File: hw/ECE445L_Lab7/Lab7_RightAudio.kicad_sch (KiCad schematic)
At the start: 60 parts, among them Q10 PZT2222A, Q11 PZT2222A, Q12 PZT2222A, Q13 PZT2222A, Q14 PZT2222A, Q15 PZT2222A, Q16 PZT2222A, Q17 PZT2222A, Q18 PZT2222A, U11 OPA2350, U12 OPA2350, U13 OPA2350, U15 TLV5616, U6 OPA2350

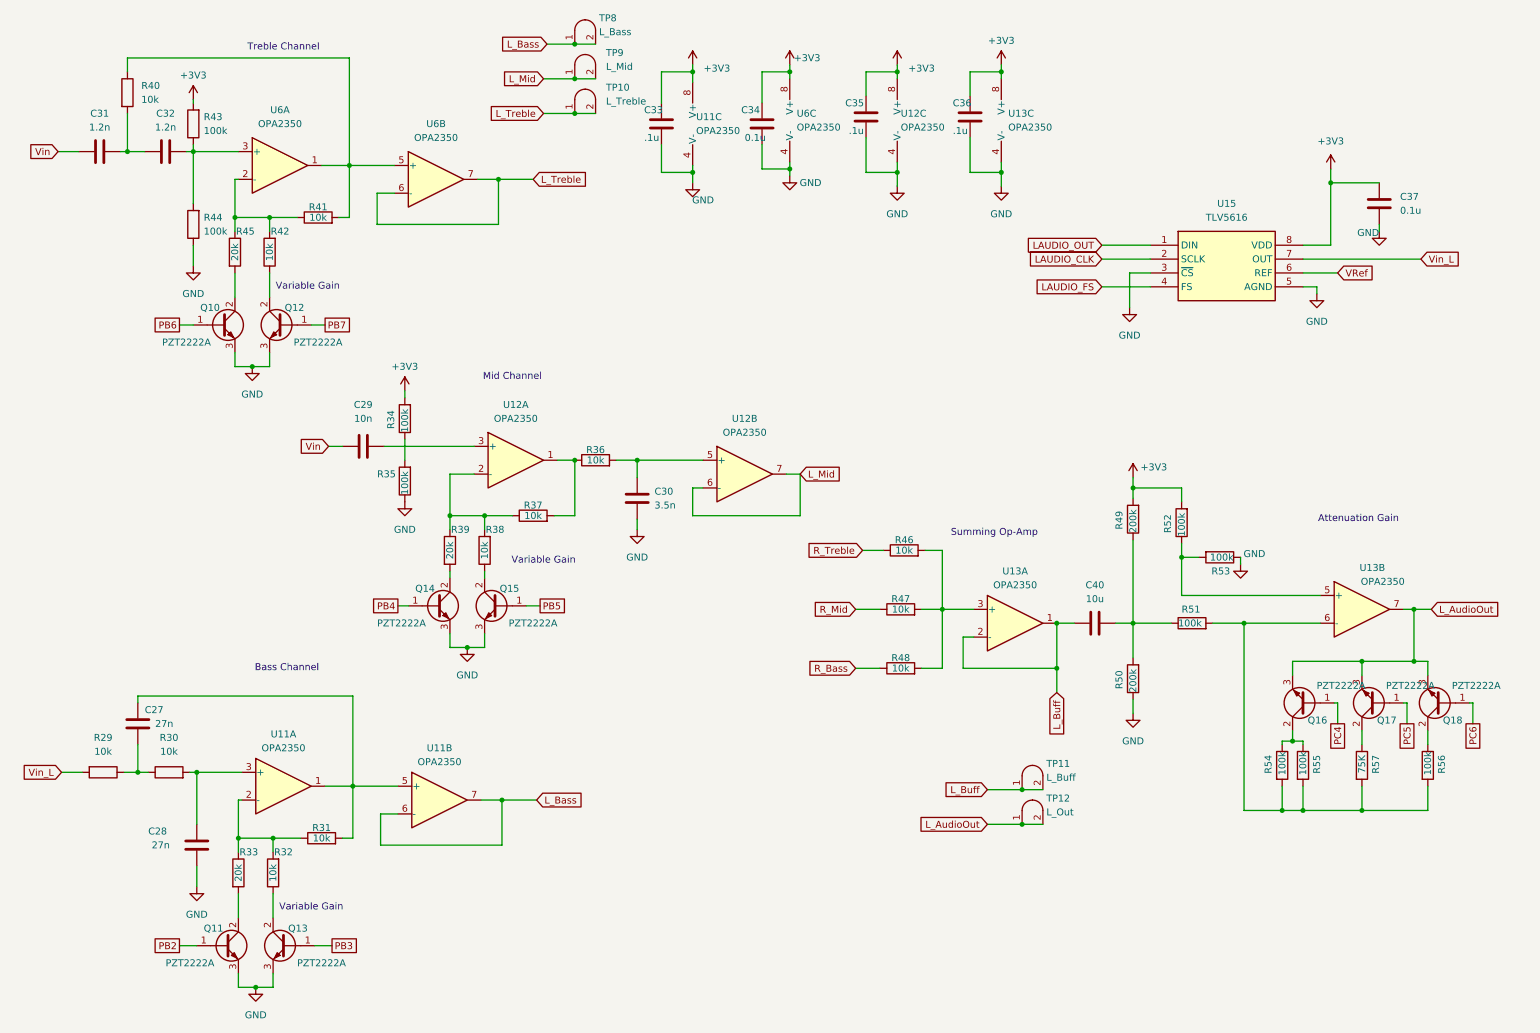
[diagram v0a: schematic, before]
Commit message: Lab7A Schematic and BOM - Ashton
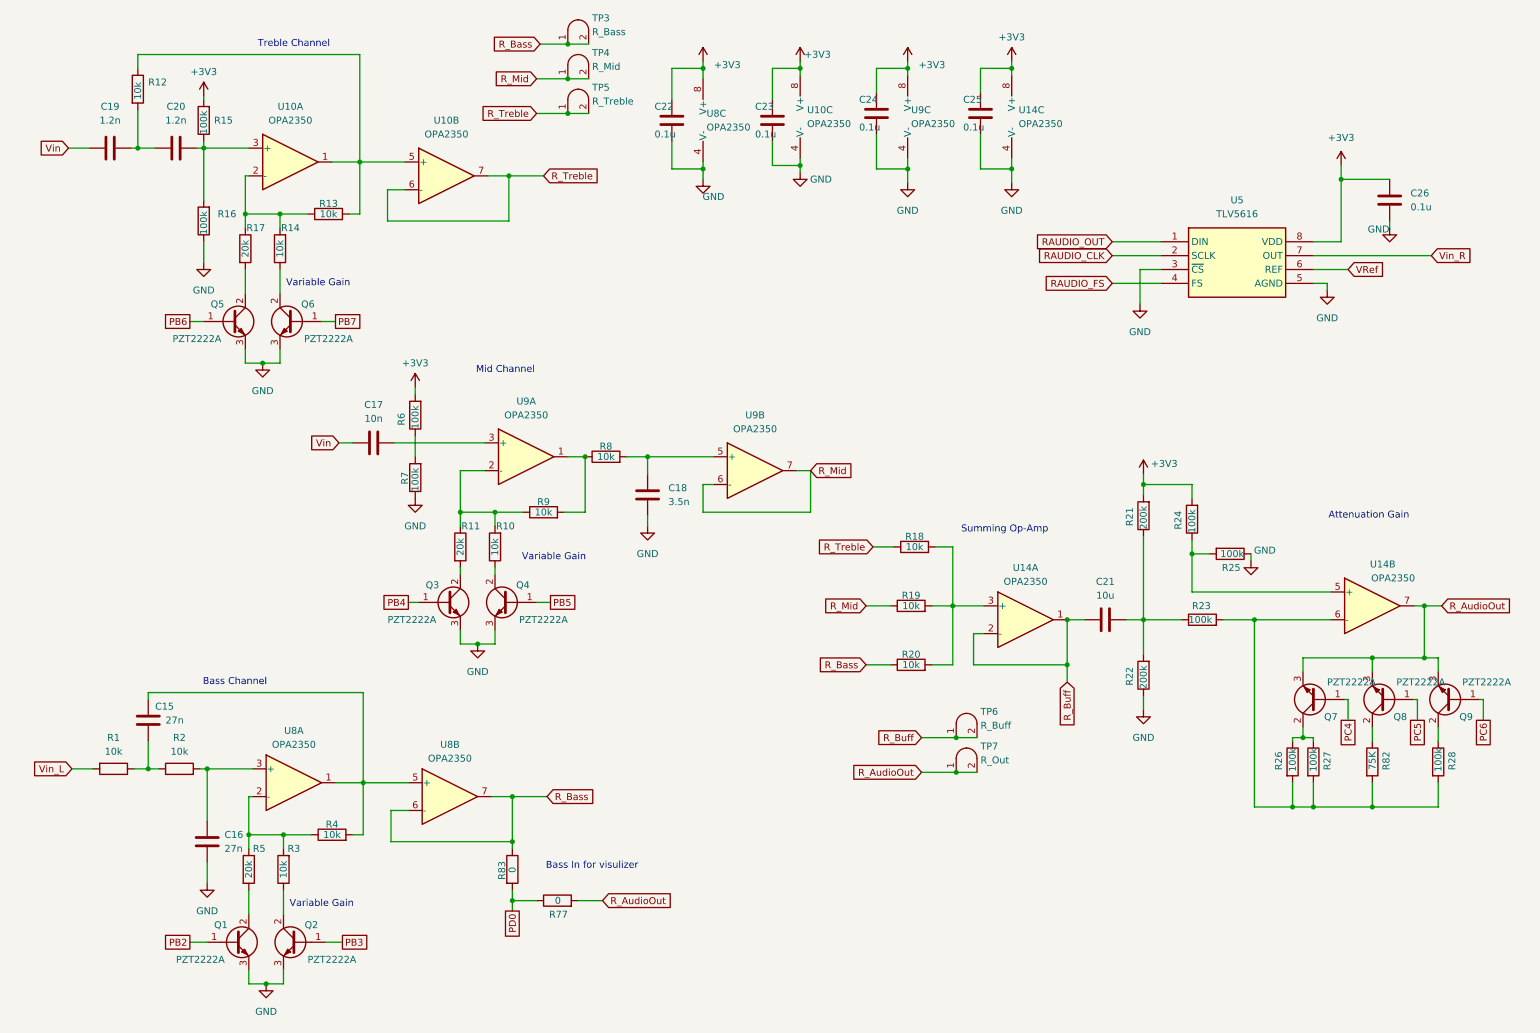
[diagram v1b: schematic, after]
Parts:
- removed C27, C28: 27n, Capacitor_SMD:C_0805_2012Metric, symbol ECE445L:C
- removed C29: 10n, Capacitor_SMD:C_0805_2012Metric, symbol ECE445L:C
- removed C30: 3.5n, Capacitor_SMD:C_0805_2012Metric, symbol ECE445L:C
- removed C31, C32: 1.2n, Capacitor_SMD:C_0805_2012Metric, symbol ECE445L:C
- removed C33, C35, C36: .1u, Capacitor_SMD:C_0805_2012Metric, symbol ECE445L:C
- removed C34: 0.1u, Capacitor_SMD:C_0805_2012Metric, symbol ECE445L:C
- removed C37: 0.1u, ECE445L:C_Axial_200mil, symbol ECE445L:C
- removed C40: 10u, Capacitor_SMD:C_0805_2012Metric, symbol ECE445L:C
- removed Q10, Q11, Q12, Q13, Q14, Q15, Q16, Q17, Q18: PZT2222A, Package_TO_SOT_SMD:SOT-223-3_TabPin2, symbol Transistor_BJT:PZT2222A
- removed R29, R30, R31, R32, R36, R37, R38, R40, R41, R42, R46, R47, R48: 10k, Resistor_SMD:R_0805_2012Metric, symbol Device:R
- removed R33, R39, R45: 20k, Resistor_SMD:R_0805_2012Metric, symbol Device:R
- removed R34, R35, R43, R44, R51, R52, R53, R54, R55, R56: 100k, Resistor_SMD:R_0805_2012Metric, symbol Device:R
- removed R49, R50: 200k, Resistor_SMD:R_0805_2012Metric, symbol Device:R
- removed R57: 75K, Resistor_SMD:R_0805_2012Metric, symbol Device:R
- removed TP10: L_Treble, ECE445L:Testpoint_1x02_P2.54mm, symbol ECE445L:Testpoint
- removed TP11: L_Buff, ECE445L:Testpoint_1x02_P2.54mm, symbol ECE445L:Testpoint
- removed TP12: L_Out, ECE445L:Testpoint_1x02_P2.54mm, symbol ECE445L:Testpoint
- removed TP8: L_Bass, ECE445L:Testpoint_1x02_P2.54mm, symbol ECE445L:Testpoint
- removed TP9: L_Mid, ECE445L:Testpoint_1x02_P2.54mm, symbol ECE445L:Testpoint
- removed U11, U12, U13, U6: OPA2350, ECE445L:DIP-8_W7.62mm_LongPads, symbol ECE445L:OPA2350
- removed U15: TLV5616, ECE445L:DIP-8_W7.62mm_LongPads, symbol ECE445L:TLV5616
- added C15, C16: 27n, Capacitor_SMD:C_0805_2012Metric, symbol ECE445L:C
- added C17: 10n, Capacitor_SMD:C_0805_2012Metric, symbol ECE445L:C
- added C18: 3.5n, Capacitor_SMD:C_0805_2012Metric, symbol ECE445L:C
- added C19, C20: 1.2n, Capacitor_SMD:C_0805_2012Metric, symbol ECE445L:C
- added C21: 10u, Capacitor_SMD:C_0805_2012Metric, symbol ECE445L:C
- added C22, C23, C24, C25: 0.1u, Capacitor_SMD:C_0805_2012Metric, symbol ECE445L:C
- added C26: 0.1u, ECE445L:C_Axial_200mil, symbol ECE445L:C
- added Q1, Q2, Q3, Q4, Q5, Q6, Q7, Q8, Q9: PZT2222A, Package_TO_SOT_SMD:SOT-223-3_TabPin2, symbol Transistor_BJT:PZT2222A
- added R1, R10, R12, R13, R14, R18, R19, R2, R20, R3, R4, R8, R9: 10k, Resistor_SMD:R_0805_2012Metric, symbol Device:R
- added R11, R17, R5: 20k, Resistor_SMD:R_0805_2012Metric, symbol Device:R
- added R15, R16, R23, R24, R25, R26, R27, R28, R6, R7: 100k, Resistor_SMD:R_0805_2012Metric, symbol Device:R
- added R21, R22: 200k, Resistor_SMD:R_0805_2012Metric, symbol Device:R
- added R77, R83: 0, symbol Device:R
- added R82: 75K, Resistor_SMD:R_0805_2012Metric, symbol Device:R
- added TP3: R_Bass, ECE445L:Testpoint_1x02_P2.54mm, symbol ECE445L:Testpoint
- added TP4: R_Mid, ECE445L:Testpoint_1x02_P2.54mm, symbol ECE445L:Testpoint
- added TP5: R_Treble, ECE445L:Testpoint_1x02_P2.54mm, symbol ECE445L:Testpoint
- added TP6: R_Buff, ECE445L:Testpoint_1x02_P2.54mm, symbol ECE445L:Testpoint
- added TP7: R_Out, ECE445L:Testpoint_1x02_P2.54mm, symbol ECE445L:Testpoint
- added U10, U14, U8, U9: OPA2350, ECE445L:DIP-8_W7.62mm_LongPads, symbol ECE445L:OPA2350
- added U5: TLV5616, ECE445L:DIP-8_W7.62mm_LongPads, symbol ECE445L:TLV5616
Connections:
- net +3V3: now also C22.2, C23.2, C24.2, C25.2, C26.1, R15.2, R21.2, R24.2, R6.2, U10.8 (V+), U14.8 (V+), U5.8 (VDD), U8.8 (V+), U9.8 (V+)
- net GND: now also C16.2, C18.1, C22.1, C23.1, C24.1, C25.1, C26.2, Q1.3 (E), Q2.3 (E), Q3.3 (E), Q4.3 (E), Q5.3 (E), Q6.3 (E), R16.1, R22.1, R25.1, R7.1, U10.4 (V-), U14.4 (V-), U5.3 (~{CS}), U5.5 (AGND), U8.4 (V-), U9.4 (V-)
- net PB2: now also Q1.1 (B)
- net PB3: now also Q2.1 (B)
- net PB4: now also Q3.1 (B)
- net PB5: now also Q4.1 (B)
- net PB6: now also Q5.1 (B)
- net PB7: now also Q6.1 (B)
- net PC4: now also Q7.1 (B)
- net PC5: now also Q8.1 (B)
- net PC6: now also Q9.1 (B)
- net R_Bass: now also R20.1, R83.1, TP3.1 (A), TP3.2 (B), U8.6 (-), U8.7
- net R_Mid: now also R19.1, TP4.1 (A), TP4.2 (B), U9.6 (-), U9.7
- net R_Treble: now also R18.1, TP5.1 (A), TP5.2 (B), U10.6 (-), U10.7
- net VRef: now also U5.6 (REF)
- net Vin: now also C17.1, C19.1
- net Vin_L: now also R1.2
- new net: Q4.2 (C), R10.1
- new net: R10.2, R11.1, R9.1, U9.2 (-)
- new net: C15.1, R4.2, U8.1, U8.5 (+)
- new net: R12.1, R13.2, U10.1, U10.5 (+)
- new net: C19.2, C20.1, R12.2
- new net: C18.2, R8.2, U9.5 (+)
- new net: Q7.2 (C), R26.1, R27.1
- new net: Q3.2 (C), R11.2
- new net: R8.1, R9.2, U9.1
- new net: C17.2, U9.3 (+)
- new net: R3.2, R4.1, R5.1, U8.2 (-)
- new net: Q1.2 (C), R5.2
- new net: C15.2, R1.1, R2.1
- new net: R24.1, R25.2, U14.5 (+)
- new net: R23.2, R26.2, R27.2, R28.2, R82.2, U14.6 (-)
- new net: Q8.2 (C), R82.1
- new net: C16.1, R2.2, U8.3 (+)
- new net: C20.2, R15.1, R16.2, U10.3 (+)
- new net: Q6.2 (C), R14.1
- new net: R13.1, R14.2, R17.1, U10.2 (-)
- new net: R18.2, R19.2, R20.2, U14.3 (+)
- new net: Q2.2 (C), R3.1
- new net: C21.2, R21.1, R22.2, R23.1
- new net: R6.1, R7.2
- new net: Q9.2 (C), R28.1
- new net: Q5.2 (C), R17.2
- new net PD0: R77.1, R83.2
- new net RAUDIO_CLK: U5.2 (SCLK)
- new net RAUDIO_FS: U5.4 (FS)
- new net RAUDIO_OUT: U5.1 (DIN)
- new net R_AudioOut: Q7.3 (E), Q8.3 (E), Q9.3 (E), R77.2, TP7.1 (A), TP7.2 (B), U14.7
- new net R_Buff: C21.1, TP6.1 (A), TP6.2 (B), U14.1, U14.2 (-)
- new net Vin_R: U5.7 (OUT)
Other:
- note added: "Bass In for visulizer"
